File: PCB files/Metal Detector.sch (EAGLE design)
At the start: 52 parts, among them IC1 NE5534AD, IC2 ESP32-WROOM-32UE-N4, IC3 CP2102, Q1 IRF740, Q2 BC556, Q3 MBT3904DW1T1, T1 BC547, X1 A1944-50

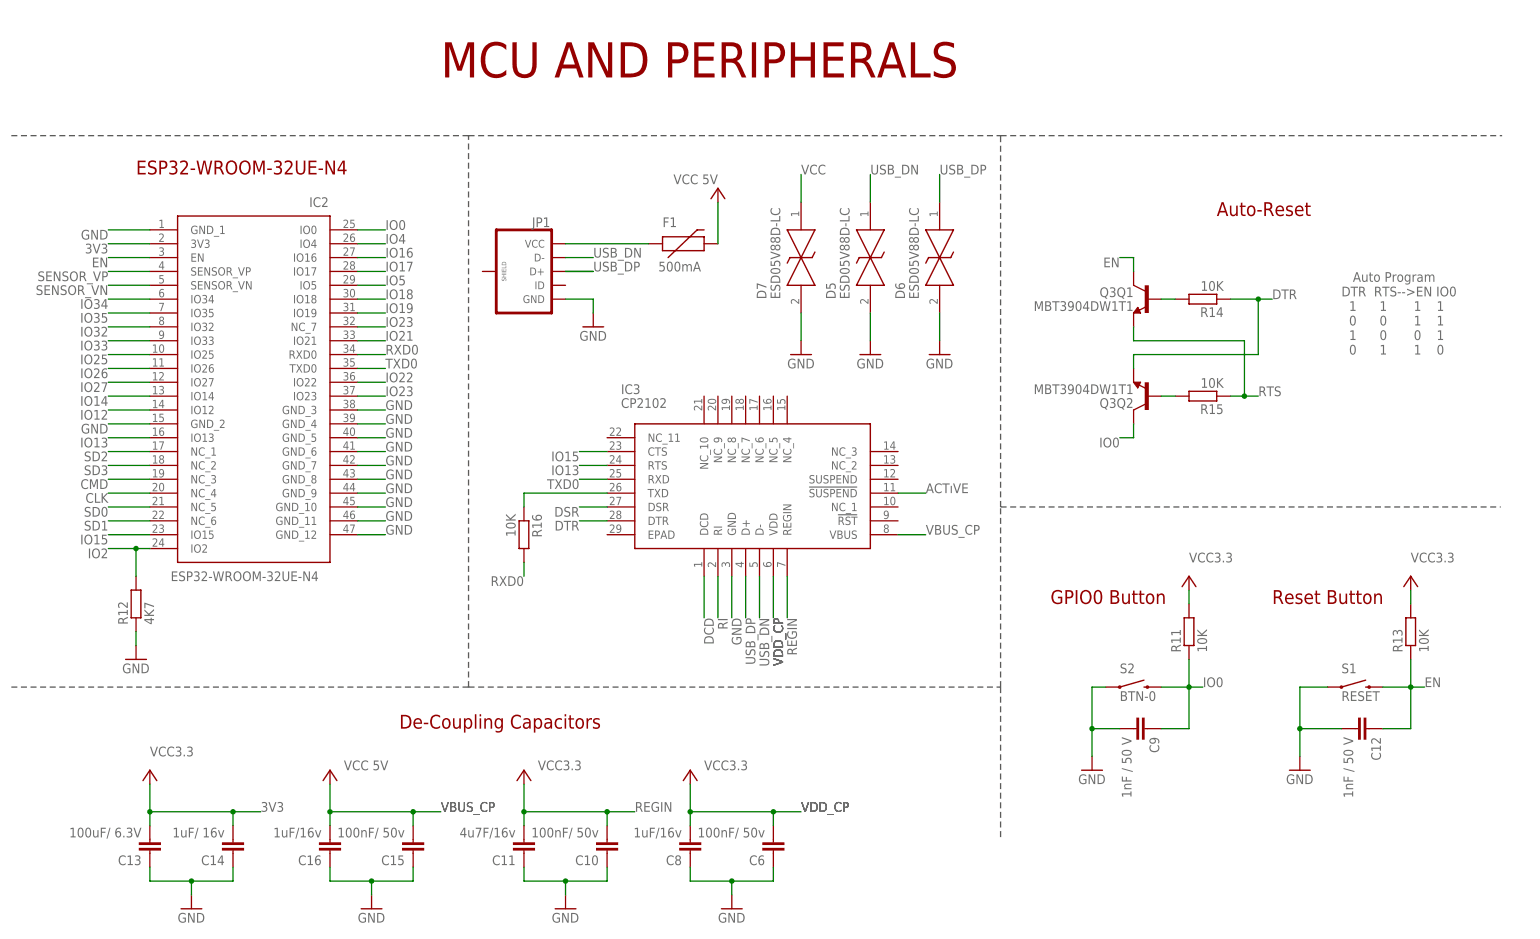
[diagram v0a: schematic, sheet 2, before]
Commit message: Add files via upload
Adding Subtitle to sheet
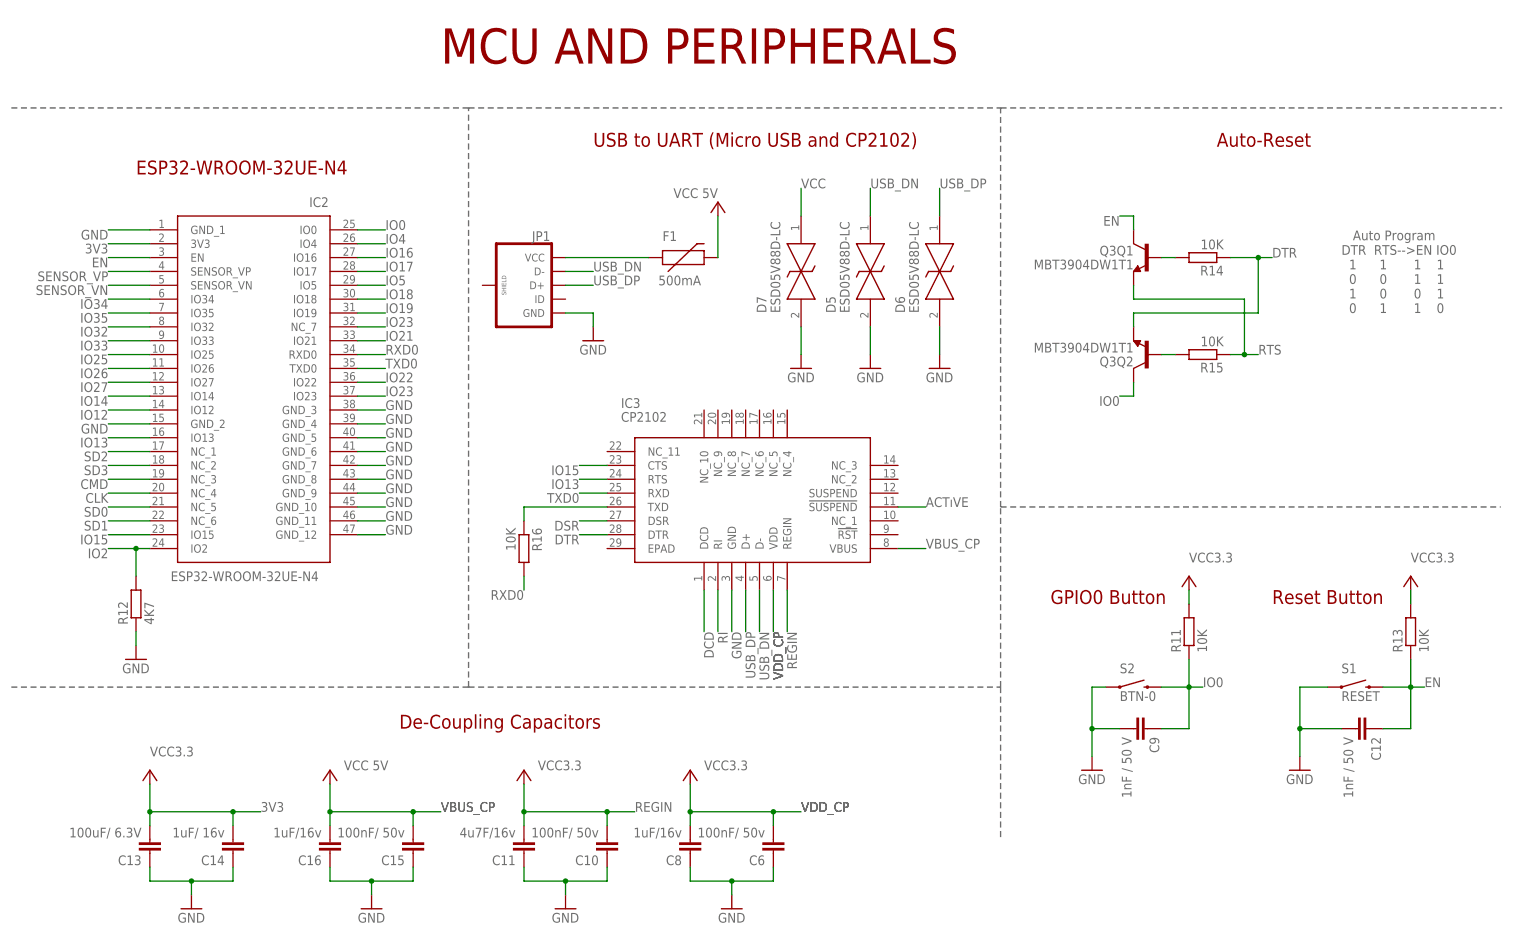
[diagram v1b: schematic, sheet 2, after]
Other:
- note added: "USB to UART (Micro USB and CP2102)"
- moved on the sheet: D5, D6, D7, F1, IC3, JP1, Q3Q1, Q3Q2, R14, R15, R16
